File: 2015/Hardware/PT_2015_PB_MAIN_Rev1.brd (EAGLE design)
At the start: 241.3 x 154.9 mm, 136 parts, among them Q1 Q_INA28, Q10 Q_INA28, Q11 Q_IRFS7437PbF, Q12 2N7002, Q13 Q_INA28, Q14 Q_IRFS7437PbF, Q15 Q_INA28, Q16 Q_IRFS7437PbF, Q17 Q_INA28, Q18 Q_IRFS7437PbF, Q19 Q_INA28, Q2 Q_INA28, Q20 Q_IRFS7437PbF, Q3 Q_INA28, Q4 Q_ACS711LC, Q5 Q_ACS711LC, Q6 Q_IRFS7437PbF, Q7 Q_IRFS7437PbF, Q8 Q_INA28, Q9 Q_IRFS7437PbF

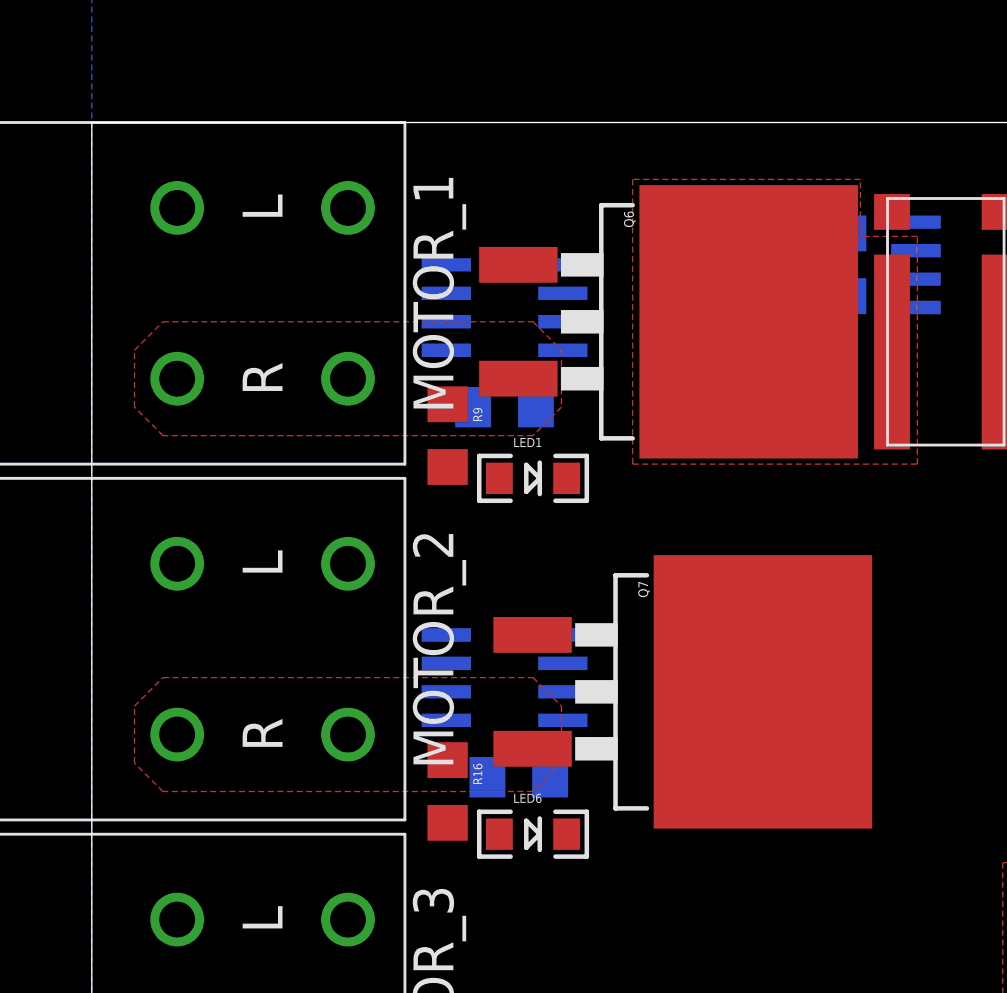
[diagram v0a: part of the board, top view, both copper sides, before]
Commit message: continued
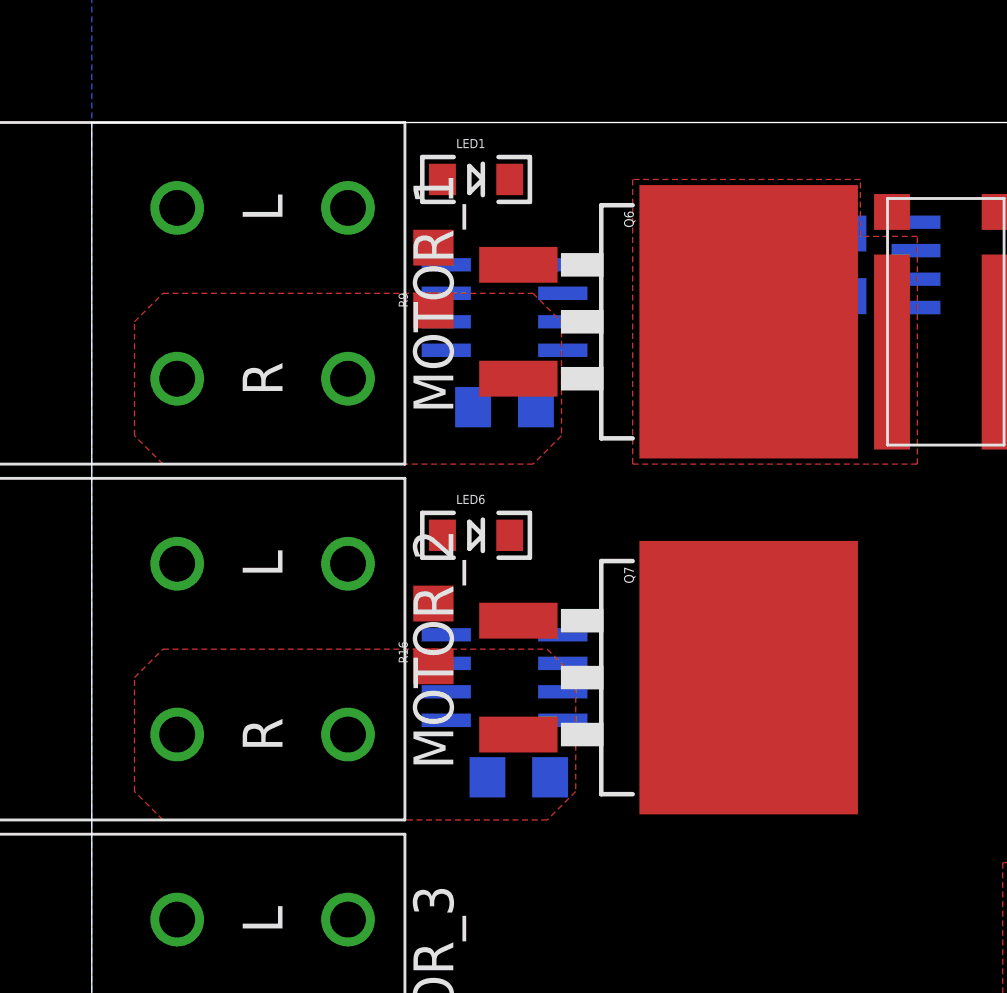
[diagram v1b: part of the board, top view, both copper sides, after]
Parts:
- moved LED1 13.6 mm to (17.1, 152.4)
- moved LED6 13.6 mm to (17.1, 136.5)
- moved R16 7.01 mm to (15.2, 132.1), turned to 90 degrees
- moved R9 7.01 mm to (15.2, 148.0), turned to 90 degrees
- moved Q7 0.90 mm to (27.3, 130.2)
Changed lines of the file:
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@@
 <element name="L7" library="MRDT-2014-All" package="L_29F0429" value="L_29F0429" x="127" y="110.49"/>
 <element name="L8" library="MRDT-2014-All" package="L_29F0429" value="L_29F0429" x="173.99" y="107.315"/>
-<element name="LED1" library="SparkFun-LED" package="LED-1206" value="" x="19.685" y="139.065"/>
+<element name="LED1" library="SparkFun-LED" package="LED-1206" value="" x="17.145" y="152.4"/>
 <element name="LED10" library="SparkFun-LED" package="LED-1206" value="" x="25.4" y="35.56"/>
 <element name="LED11" library="SparkFun-LED" package="LED-1206" value="" x="25.4" y="-10.16"/>
@@
 <element name="LED4" library="SparkFun-LED" package="LED-1206" value="" x="235.585" y="111.125" rot="R180"/>
 <element name="LED5" library="SparkFun-LED" package="LED-1206" value="" x="235.585" y="60.96"/>
-<element name="LED6" library="SparkFun-LED" package="LED-1206" value="" x="19.685" y="123.19"/>
+<element name="LED6" library="SparkFun-LED" package="LED-1206" value="" x="17.145" y="136.525"/>
 <element name="LED7" library="SparkFun-LED" package="LED-1206" value="" x="25.4" y="104.14"/>
 <element name="LED8" library="SparkFun-LED" package="LED-1206" value="" x="25.4" y="81.28"/>
@@
 <element name="Q5" library="MRDT-2015-PowerBoard" package="SOIC8_ACS711" value="Q_ACS711LC" x="222.885" y="73.66" rot="R180"/>
 <element name="Q6" library="MRDT-2015-PowerBoard" package="D2PACK" value="Q_IRFS7437PbF" x="27.305" y="146.05" rot="R270"/>
-<element name="Q7" library="MRDT-2015-PowerBoard" package="D2PACK" value="Q_IRFS7437PbF" x="27.94" y="129.54" rot="R270"/>
+<element name="Q7" library="MRDT-2015-PowerBoard" package="D2PACK" value="Q_IRFS7437PbF" x="27.305" y="130.175" rot="R270"/>
 <element name="Q8" library="MRDT-2014-All" package="SOIC8" value="Q_INA28" x="55.88" y="102.87" rot="R180"/>
 <element name="Q9" library="MRDT-2015-PowerBoard" package="D2PACK" value="Q_IRFS7437PbF" x="43.18" y="92.71" rot="R270"/>
@@
 <element name="R14" library="MRDT-2014-All" package="R_FC4L" value=".001Ω" x="55.88" y="115.57"/>
 <element name="R15" library="resistor" package="R1206" value="" x="65.405" y="113.665" rot="R180"/>
-<element name="R16" library="SparkFun-Passives" package="1206" value="1kΩ" x="15.875" y="125.095" rot="R270"/>
+<element name="R16" library="SparkFun-Passives" package="1206" value="1kΩ" x="15.24" y="132.08" rot="R90"/>
 <element name="R17" library="MRDT-2014-All" package="R_FC4L" value=".001Ω" x="55.88" y="92.71"/>
 <element name="R18" library="SparkFun-Passives" package="1206" value="1kΩ" x="19.685" y="104.14"/>
@@
 <element name="R7" library="resistor" package="R1206" value="585Ω" x="203.2" y="85.09"/>
 <element name="R8" library="resistor" package="R1206" value="21kΩ" x="192.405" y="109.22"/>
-<element name="R9" library="SparkFun-Passives" package="1206" value="1kΩ" x="15.875" y="140.97" rot="R270"/>
+<element name="R9" library="SparkFun-Passives" package="1206" value="1kΩ" x="15.24" y="147.955" rot="R90"/>
 <element name="SIDEOUS-12V" library="MRDT-2015-PowerBoard" package="U-T48-QB-NO_TRIM" value="UQW-12/20-T48NBS" x="92.075" y="135.255" rot="R180"/>
 <element name="U$1" library="MRDT-2015-General" package="32U4_MCU_DIP" value="32U4_BREAKOUT" x="205.74" y="48.895" rot="R270"/>
@@
 <wire x1="176.53" y1="135.76" x2="176.84" y2="131.45" width="0" layer="19" extent="1-1"/>
 <wire x1="180.28" y1="137.795" x2="176.53" y2="135.76" width="0" layer="19" extent="1-1"/>
-<wire x1="21.185" y1="123.19" x2="17.65" y2="125.73" width="0" layer="19" extent="1-16"/>
 <wire x1="185.48" y1="137.795" x2="180.28" y2="137.795" width="0" layer="19" extent="1-1"/>
 <wire x1="189.23" y1="138.56" x2="185.48" y2="137.795" width="0" layer="19" extent="1-1"/>
-<wire x1="21.185" y1="139.065" x2="17.015" y2="142.24" width="0" layer="19" extent="1-16"/>
 <wire x1="222.885" y1="112.9" x2="220.98" y2="107.95" width="0" layer="19" extent="1-1"/>
 <wire x1="226.06" y1="113.82" x2="222.885" y2="112.9" width="0" layer="19" extent="1-1"/>
 <wire x1="237.085" y1="60.96" x2="233.68" y2="65.52" width="0" layer="19" extent="1-1"/>
 <wire x1="220.98" y1="71.06" x2="217.805" y2="66.17" width="0" layer="19" extent="1-1"/>
+<wire x1="18.645" y1="136.525" x2="17.015" y2="142.24" width="0" layer="19" extent="1-16"/>
 <wire x1="170.815" y1="133.855" x2="176.53" y2="135.76" width="0" layer="19" extent="1-1"/>
 <wire x1="226.695" y1="66.17" x2="233.68" y2="65.52" width="0" layer="19" extent="1-1"/>
+<wire x1="18.645" y1="152.4" x2="11.43" y2="151.13" width="0" layer="19" extent="1-1"/>
 <wire x1="236.45" y1="81.915" x2="233.68" y2="74.41" width="0" layer="19" extent="1-1"/>
 <wire x1="234.085" y1="111.125" x2="233.68" y2="102.985" width="0" layer="19" extent="1-1"/>
@@
 <contactref element="R9" pad="1"/>
 <polygon width="0.4064" layer="1" thermals="no">
-<vertex x="20.955" y="144.78"/>
-<vertex x="20.955" y="142.24"/>
-<vertex x="19.685" y="140.97"/>
-<vertex x="3.175" y="140.97"/>
-<vertex x="1.905" y="142.24"/>
-<vertex x="1.905" y="144.78"/>
-<vertex x="3.175" y="146.05"/>
-<vertex x="19.685" y="146.05"/>
+<vertex x="20.955" y="146.05"/>
+<vertex x="20.955" y="140.97"/>
+<vertex x="19.685" y="139.7"/>
+<vertex x="3.175" y="139.7"/>
+<vertex x="1.905" y="140.97"/>
+<vertex x="1.905" y="146.05"/>
+<vertex x="3.175" y="147.32"/>
+<vertex x="19.685" y="147.32"/>
 </polygon>
 </signal>
@@
 <contactref element="R9" pad="2"/>
 <contactref element="LED1" pad="A"/>
-<wire x1="15.875" y1="139.57" x2="18.185" y2="139.065" width="0" layer="19" extent="1-1"/>
+<wire x1="15.24" y1="149.355" x2="15.645" y2="152.4" width="0" layer="19" extent="1-1"/>
 </signal>
 <signal name="N$46">
@@
 <vertex x="52.07" y="119.38"/>
 </polygon>
-<wire x1="21.015" y1="130.81" x2="29.94" y2="129.54" width="0" layer="19" extent="1-16"/>
+<wire x1="21.015" y1="130.81" x2="29.305" y2="130.175" width="0" layer="19" extent="1-16"/>
 <wire x1="21.015" y1="128.27" x2="21.015" y2="130.81" width="0" layer="19" extent="16-16"/>
 <wire x1="20.45" y1="125.73" x2="21.015" y2="128.27" width="0" layer="19" extent="16-16"/>
-<wire x1="53.48" y1="114.22" x2="29.94" y2="129.54" width="0" layer="19" extent="1-1"/>
+<wire x1="53.48" y1="114.22" x2="29.305" y2="130.175" width="0" layer="19" extent="1-1"/>
 </signal>
 <signal name="N$29">
@@
 <contactref element="R16" pad="1"/>
 <polygon width="0.4064" layer="1" thermals="no">
-<vertex x="20.955" y="128.905"/>
-<vertex x="20.955" y="126.365"/>
-<vertex x="19.685" y="125.095"/>
-<vertex x="3.175" y="125.095"/>
-<vertex x="1.905" y="126.365"/>
-<vertex x="1.905" y="128.905"/>
-<vertex x="3.175" y="130.175"/>
-<vertex x="19.685" y="130.175"/>
+<vertex x="21.59" y="130.175"/>
+<vertex x="21.59" y="125.095"/>
+<vertex x="20.32" y="123.825"/>
+<vertex x="3.175" y="123.825"/>
+<vertex x="1.905" y="125.095"/>
+<vertex x="1.905" y="130.175"/>
+<vertex x="3.175" y="131.445"/>
+<vertex x="20.32" y="131.445"/>
 </polygon>
 </signal>
@@
 <contactref element="Q7" pad="1"/>
 <contactref element="U$7" pad="5"/>
-<wire x1="19.665" y1="132.08" x2="21.015" y2="132.08" width="0" layer="19" extent="1-16"/>
+<wire x1="19.03" y1="132.715" x2="21.015" y2="132.08" width="0" layer="19" extent="1-16"/>
 </signal>
 <signal name="N$31">
 <contactref element="R16" pad="2"/>
 <contactref element="LED6" pad="A"/>
-<wire x1="15.875" y1="123.695" x2="18.185" y2="123.19" width="0" layer="19" extent="1-1"/>
+<wire x1="15.24" y1="133.48" x2="15.645" y2="136.525" width="0" layer="19" extent="1-1"/>
 </signal>
 <signal name="N$32">
